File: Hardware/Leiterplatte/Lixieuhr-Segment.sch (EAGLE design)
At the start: 13 parts, among them U1 APA102C, U10 APA102C, U2 APA102C, U3 APA102C, U4 APA102C, U5 APA102C, U6 APA102C, U7 APA102C, U8 APA102C, U9 APA102C

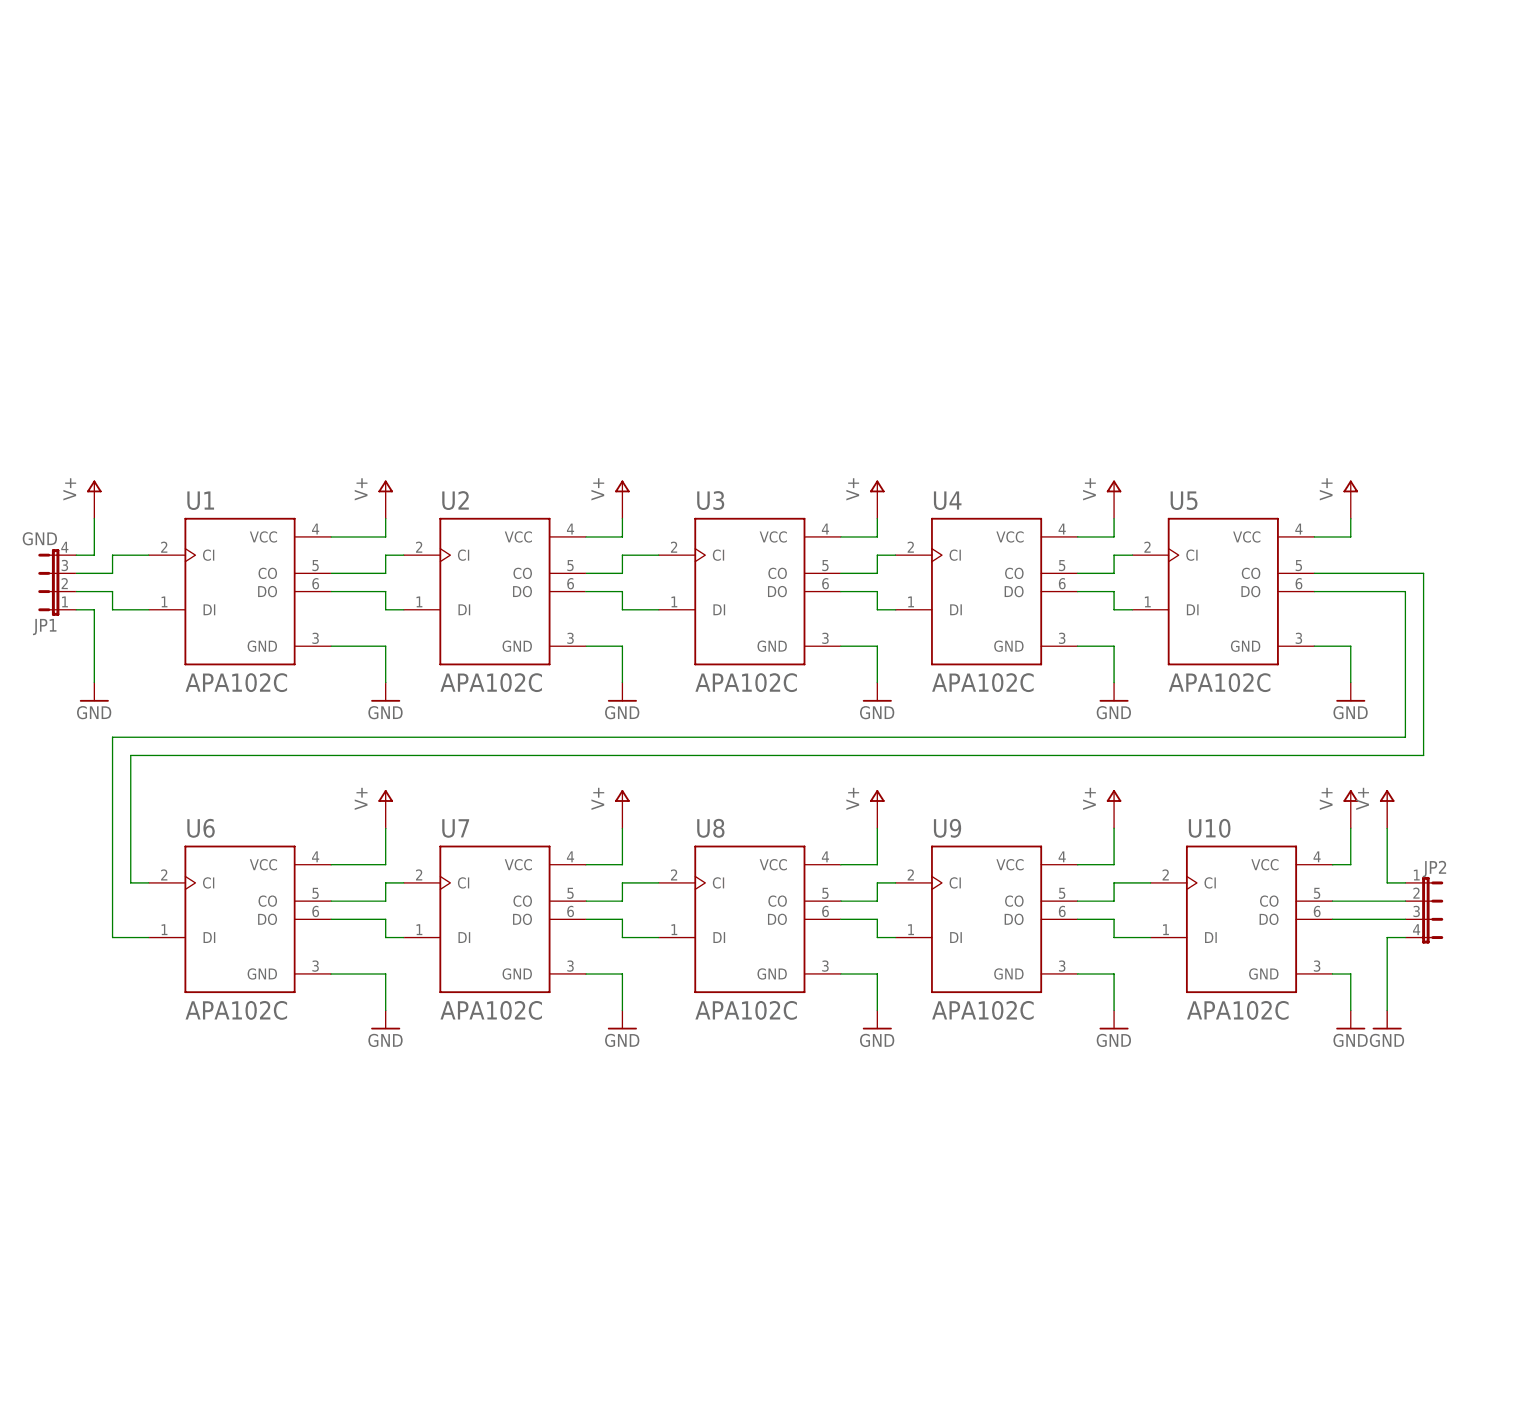
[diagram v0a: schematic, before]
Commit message: Schaltpläne V02
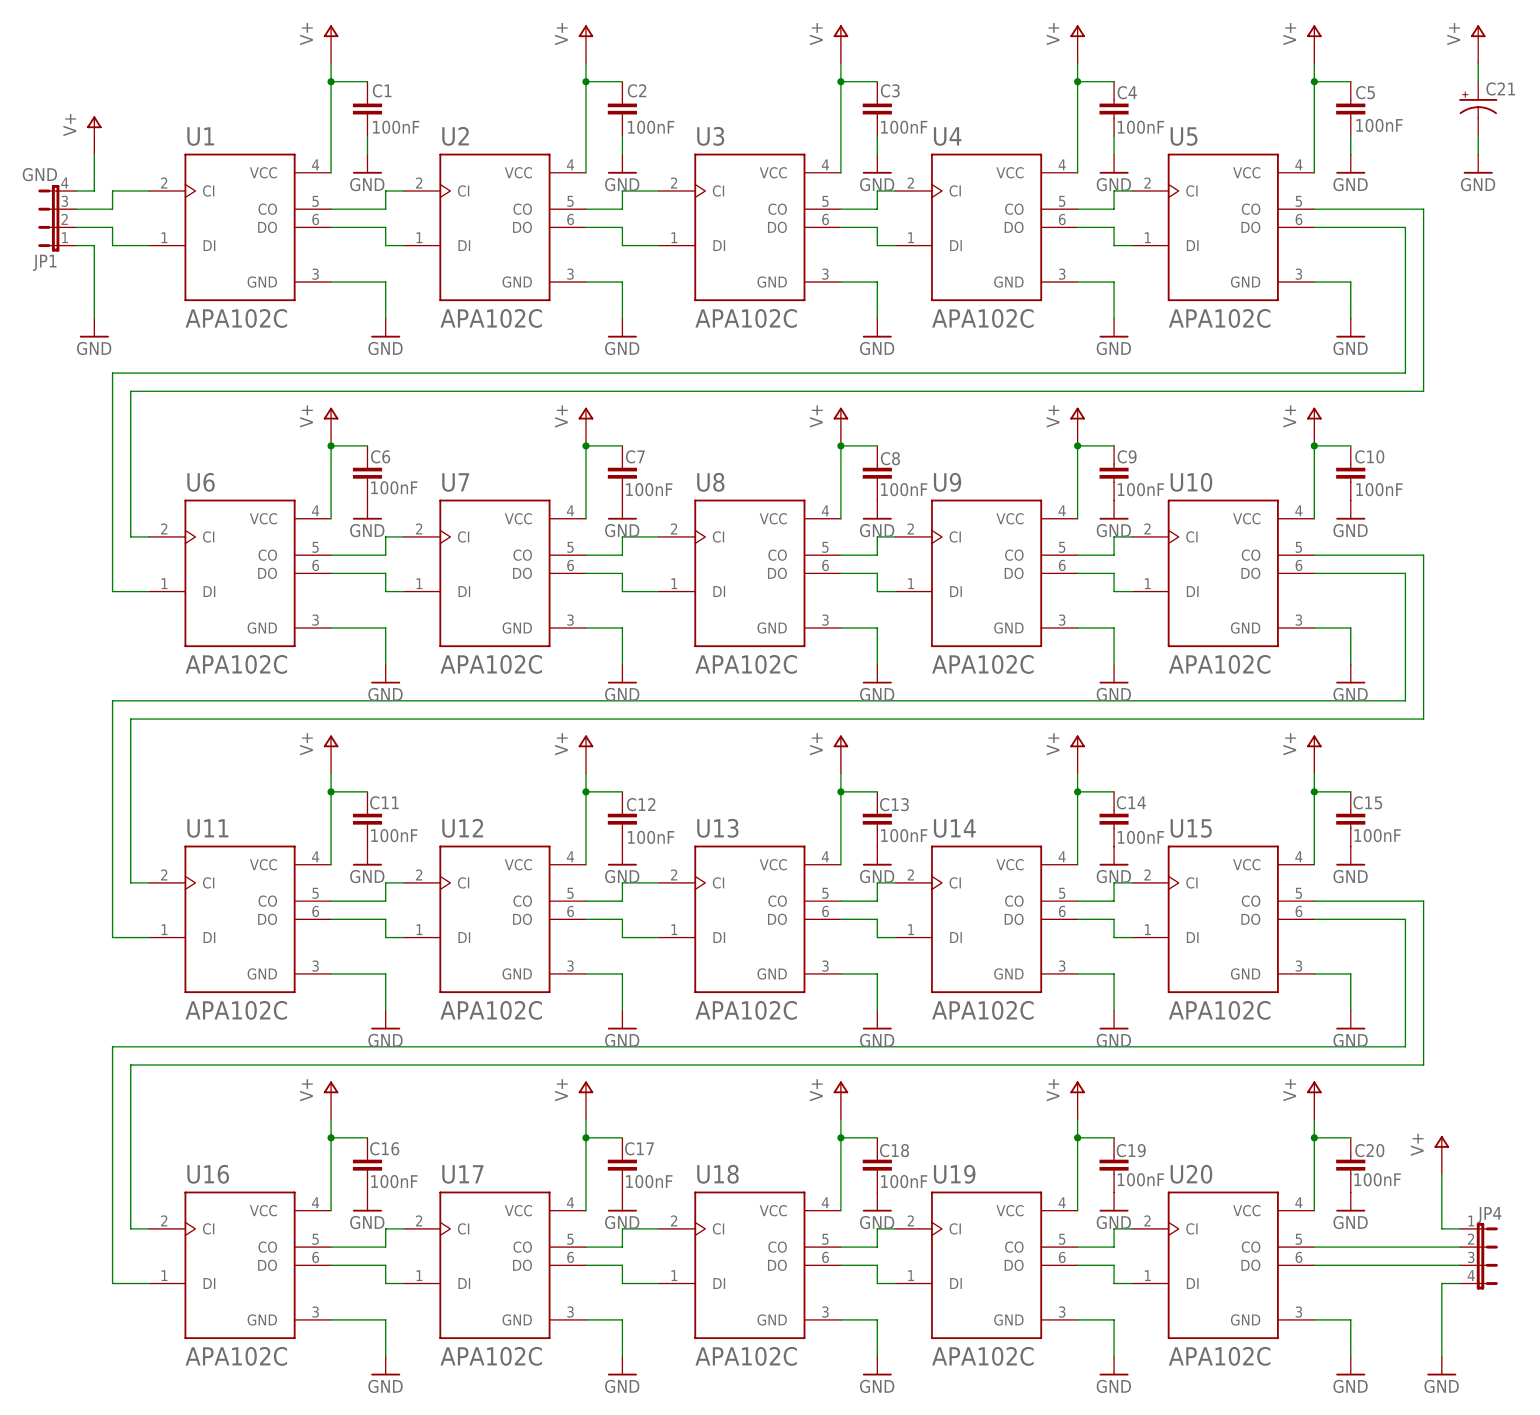
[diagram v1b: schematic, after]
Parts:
- removed FRAME1: HTL-A4-HA4H, 0_HTL_frame:HTL-A4-HA4H
- removed JP2: (no value), jumper:JP4E
- added C1, C10, C11, C12, C13, C14, C15, C16, C17, C18, C19, C2, C20, C3, C4, C5, C6, C7, C8, C9: 100nF, 0_HTL_MegaCard_V3:C-0805
- added C21: (no value), rcl:CPOL-USE3.5-8
- added JP4: (no value), jumper:JP4E
- added U11, U12, U13, U14, U15, U16, U17, U18, U19, U20: APA102C, APA102C:APA102C
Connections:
- new net N$23: U11.CO, U12.CI
- new net N$24: U12.CO, U13.CI
- new net N$25: U13.CO, U14.CI
- new net N$26: U14.CO, U15.CI
- new net N$27: U16.CO, U17.CI
- new net N$28: U17.CO, U18.CI
- new net N$29: U18.CO, U19.CI
- new net N$30: U19.CO, U20.CI
- new net N$31: U11.DO, U12.DI
- new net N$32: U12.DO, U13.DI
- new net N$33: U13.DO, U14.DI
- new net N$34: U14.DO, U15.DI
- new net N$36: U19.DO, U20.DI
- new net N$37: U16.DO, U17.DI
- new net N$38: U17.DO, U18.DI
- new net N$39: U18.DO, U19.DI
- new net N$43: JP4.2, U20.CO
- new net N$44: JP4.3, U20.DO
- new net N$47: U15.CO, U16.CI
- new net N$48: U15.DO, U16.DI
- net GND: now also C1.1, C10.1, C11.1, C12.1, C13.1, C14.1, C15.1, C16.1, C17.1, C18.1, C19.1, C2.1, C20.1, C21.-, C3.1, C4.1, C5.1, C6.1, C7.1, C8.1, C9.1, JP4.4, U11.GND, U12.GND, U13.GND, U14.GND, U15.GND, U16.GND, U17.GND, U18.GND, U19.GND, U20.GND; no longer JP2.4
- net N$21: now also U11.CI; no longer JP2.2
- net N$22: now also U11.DI; no longer JP2.3
- net V+: now also C1.2, C10.2, C11.2, C12.2, C13.2, C14.2, C15.2, C16.2, C17.2, C18.2, C19.2, C2.2, C20.2, C21.+, C3.2, C4.2, C5.2, C6.2, C7.2, C8.2, C9.2, JP4.1, U11.VCC, U12.VCC, U13.VCC, U14.VCC, U15.VCC, U16.VCC, U17.VCC, U18.VCC, U19.VCC, U20.VCC; no longer JP2.1
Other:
- note added: "Lixie-Uhr-Slave"
- note removed: "Lixie-Uhr"
- moved on the sheet: JP1, U1, U10, U2, U3, U4, U5, U6, U7, U8, U9
